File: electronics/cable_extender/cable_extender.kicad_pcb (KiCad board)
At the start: 2 copper layers, 28.8 x 31.7 mm, 10 parts, among them J1 Conn_01x11, J2 Conn_01x06, J3 Conn_01x06, J4 Conn_01x11, J5 Conn_01x11, J6 Conn_01x11, J7 Conn_01x13, J8 Conn_01x13

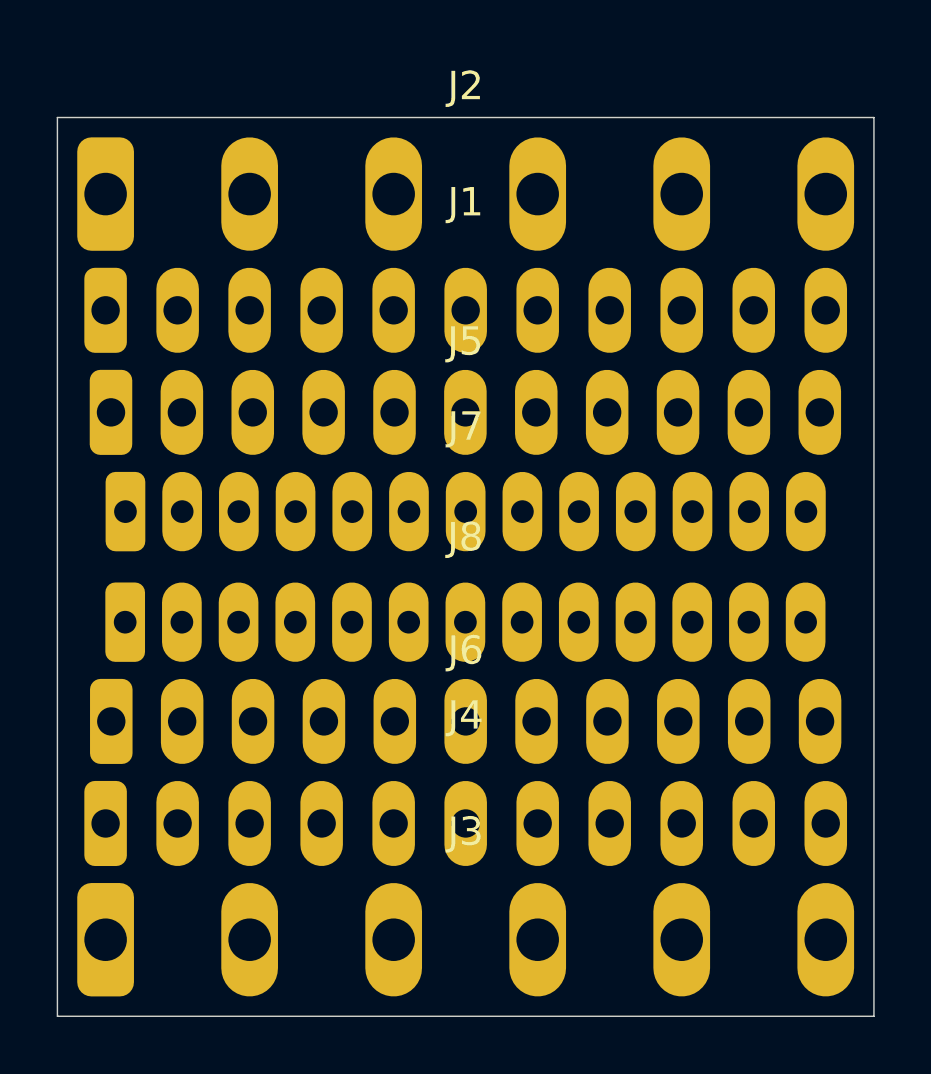
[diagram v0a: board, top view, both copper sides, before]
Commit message: routing completed
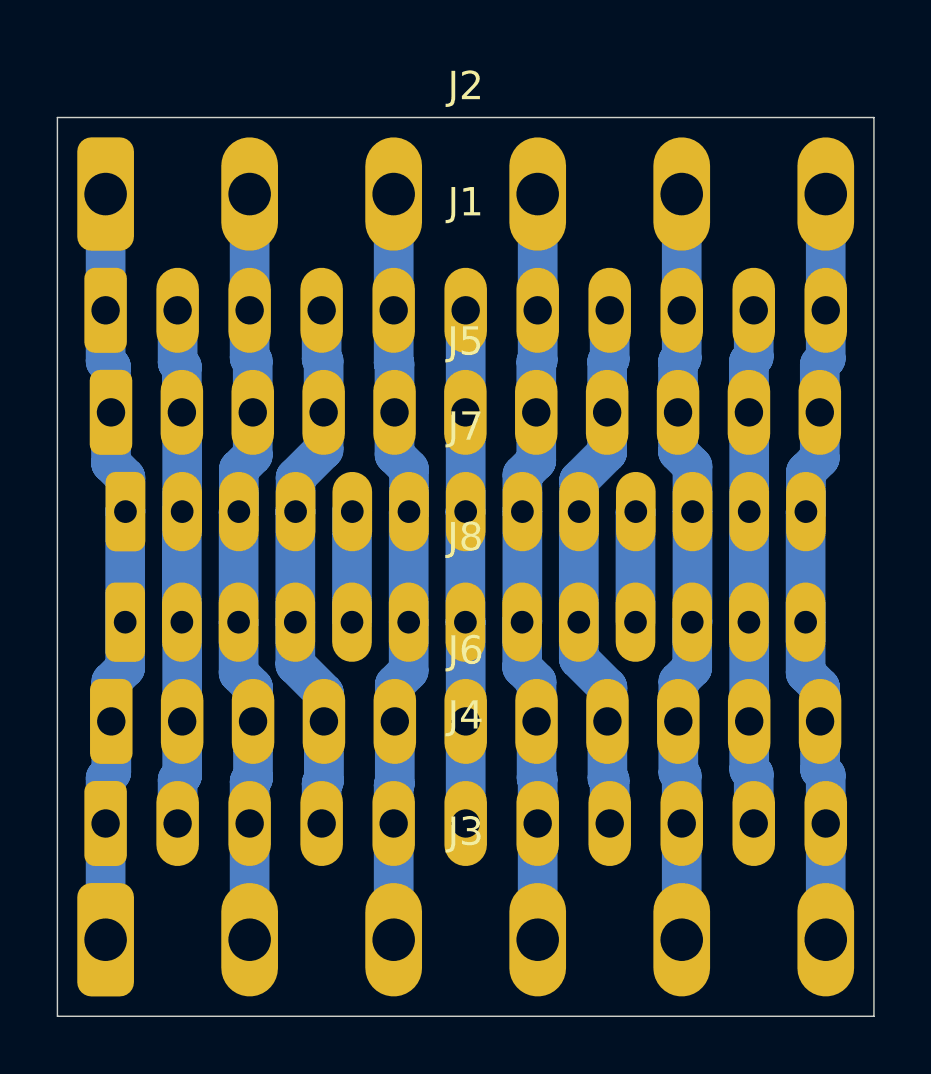
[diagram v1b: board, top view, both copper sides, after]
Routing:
- net /PIN_13: track 0.00 -> 26.9 mm
- net /PIN_01: track 0.00 -> 26.9 mm
- net /PIN_11: track 0.00 -> 26.8 mm
- net /PIN_03: track 0.00 -> 26.8 mm
- net /PIN_08: track 0.00 -> 26.8 mm
- net /PIN_06: track 0.00 -> 26.7 mm
- net /PIN_09: track 0.00 -> 19.0 mm
- net /PIN_04: track 0.00 -> 19.0 mm
- net /PIN_12: track 0.00 -> 18.2 mm
- net /PIN_02: track 0.00 -> 18.2 mm
- net /PIN_07: track 0.00 -> 18.1 mm
- net /PIN_10: track 0.00 -> 3.90 mm
- net /PIN_05: track 0.00 -> 3.90 mm
